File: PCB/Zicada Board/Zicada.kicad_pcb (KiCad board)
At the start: 2 copper layers, 57.4 x 12 mm, 60 parts, among them J1 Conn_ARM_JTAG_SWD_10, J2 Conn_01x01_Pin, J3 Conn_01x01_Pin, SW1 SW_Push, U1 nRF52840, U2 HDC2080, U3 SM351LT, U4 TPS610981, U5 OPT3001, Y1 32MHz, Y2 32.768kHz

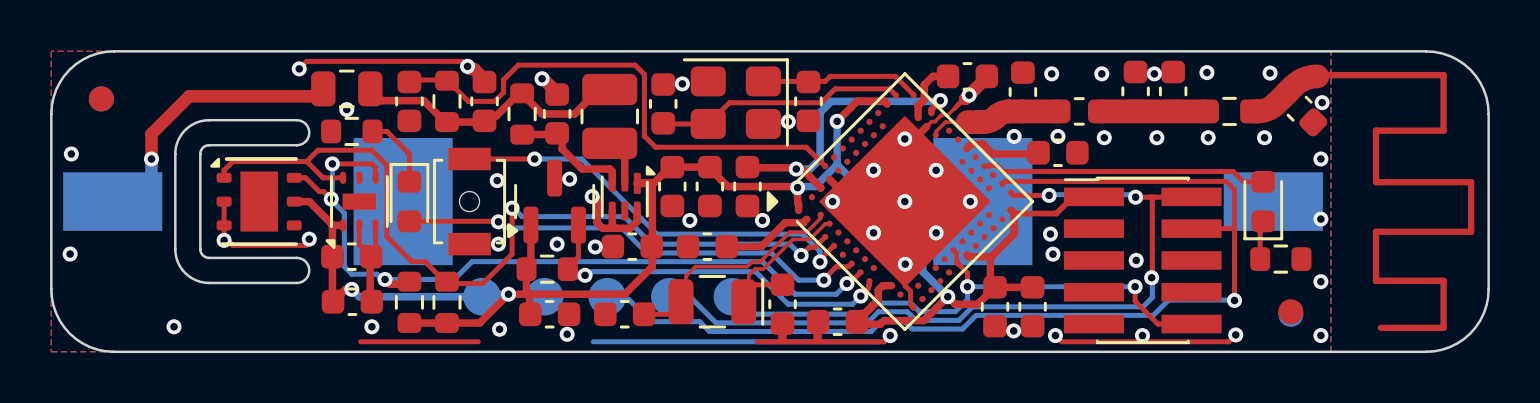
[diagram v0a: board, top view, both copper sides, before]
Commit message: generated fabrication files
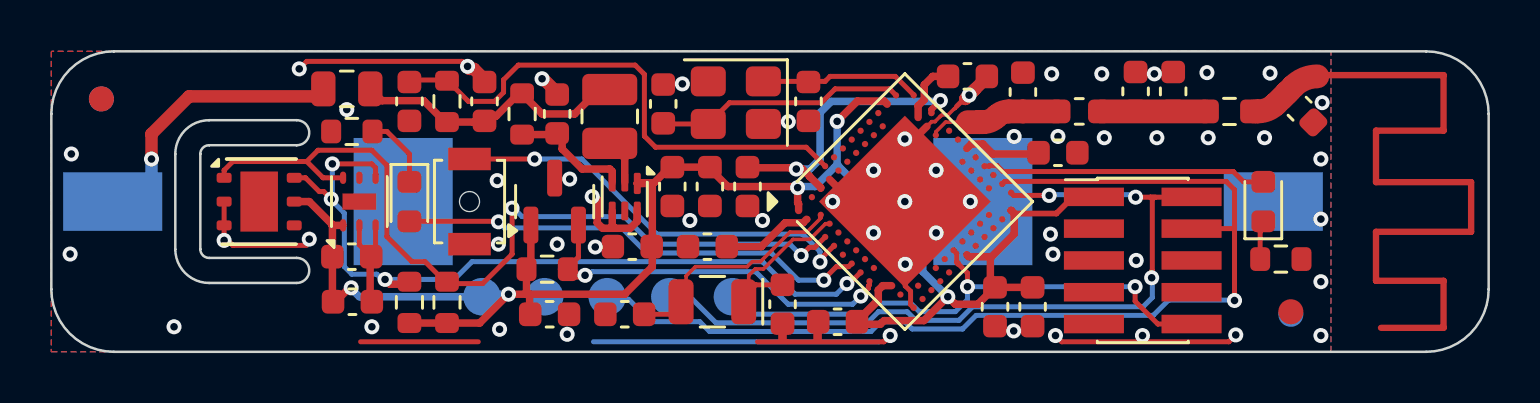
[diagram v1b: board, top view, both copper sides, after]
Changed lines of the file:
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@@
 			)
 		)
-		(property "LCSC" "C3761461"
+		(property "LCSC" "C207021"
 			(at 0 0 180)
 			(unlocked yes)
@@
 			)
 		)
+		(property "LCSC" "C90462"
+			(at 0 0 90)
+			(unlocked yes)
+			(layer "F.Fab")
+			(hide yes)
+			(effects
+				(font
+					(size 1 1)
+					(thickness 0.15)
+				)
+			)
+		)
 		(property ki_fp_filters "Lite*On*LTR*303ALS*01*")
 		(sheetname "/")
@@
 			(net 79 "unconnected-(U5-INT-Pad5)")
 			(pinfunction "INT")
-			(pintype "open_collector")
+			(pintype "open_collector+no_connect")
 		)
 		(pad "6" smd roundrect
@@
 	)
 	(segment
+		(start 134.774989 96.444426)
+		(end 134.705574 96.444426)
+		(width 0.3)
+		(layer "F.Cu")
+		(net 3)
+	)
+	(segment
 		(start 146.2 92.275)
 		(end 146.225 92.25)
@@
 	)
 	(segment
-		(start 134.8 96.504943)
-		(end 134.545057 96.504943)
-		(width 0.3)
-		(layer "F.Cu")
-		(net 3)
-	)
-	(segment
 		(start 145.7 96.7)
 		(end 141.9 96.7)
@@
 	)
 	(segment
+		(start 134.15 97)
+		(end 134.05 97)
+		(width 0.3)
+		(layer "F.Cu")
+		(net 3)
+	)
+	(segment
 		(start 134.05 97)
 		(end 134.025 97)
@@
 	)
 	(segment
+		(start 134.705574 96.444426)
+		(end 134.15 97)
+		(width 0.3)
+		(layer "F.Cu")
+		(net 3)
+	)
+	(segment
 		(start 152.55997 92.4)
 		(end 149.814266 92.4)
@@
 	)
 	(segment
-		(start 134.545057 96.504943)
-		(end 134.05 97)
-		(width 0.3)
-		(layer "F.Cu")
-		(net 3)
-	)
-	(segment
 		(start 161.252907 94.295075)
 		(end 160.347982 95.2)
@@
 	)
 	(via
-		(at 134.8 96.504943)
+		(at 134.774989 96.444426)
 		(size 0.6)
 		(drill 0.3)
@@
 	)
 	(segment
+		(start 134.774989 96.474989)
+		(end 135.1 96.8)
+		(width 0.3)
+		(layer "B.Cu")
+		(net 3)
+	)
+	(segment
 		(start 152.646188 92.4)
 		(end 153.305995 92.4)
@@
 	)
 	(segment
+		(start 135.1 96.8)
+		(end 140 96.8)
+		(width 0.3)
+		(layer "B.Cu")
+		(net 3)
+	)
+	(segment
 		(start 141.056694 96.7)
 		(end 140.1 96.7)
@@
 	)
 	(segment
-		(start 135.095057 96.8)
-		(end 140 96.8)
-		(width 0.3)
-		(layer "B.Cu")
-		(net 3)
-	)
-	(segment
 		(start 154.25 91.6)
 		(end 154.180995 91.530995)
@@
 	)
 	(segment
-		(start 158.6 96.8)
-		(end 157.6 95.8)
+		(start 134.774989 96.444426)
+		(end 134.774989 96.474989)
 		(width 0.3)
 		(layer "B.Cu")
@@
 	)
 	(segment
-		(start 134.8 96.504943)
-		(end 135.095057 96.8)
+		(start 158.6 96.8)
+		(end 157.6 95.8)
 		(width 0.3)
 		(layer "B.Cu")
